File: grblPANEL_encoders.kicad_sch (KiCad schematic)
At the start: 28 parts, among them J701 Conn_01x04, J702 Conn_01x04, J703 Conn_01x04, J704 Conn_01x04

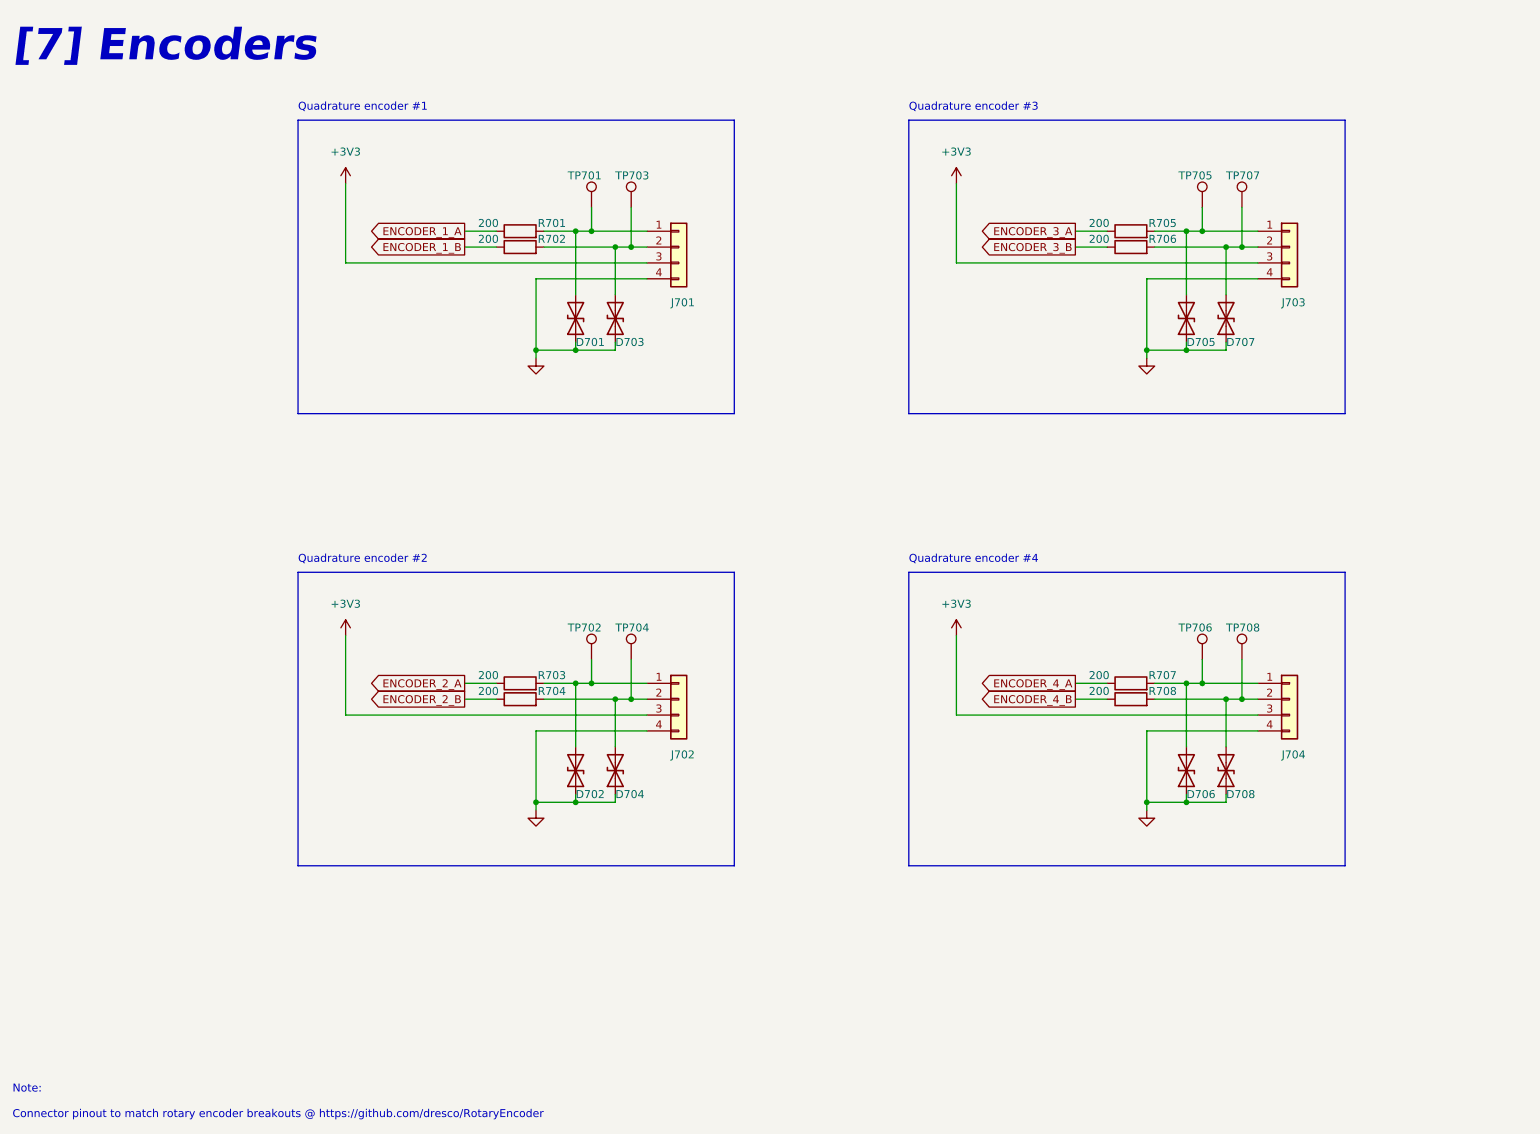
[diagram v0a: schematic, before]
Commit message: PCB layout - WIP
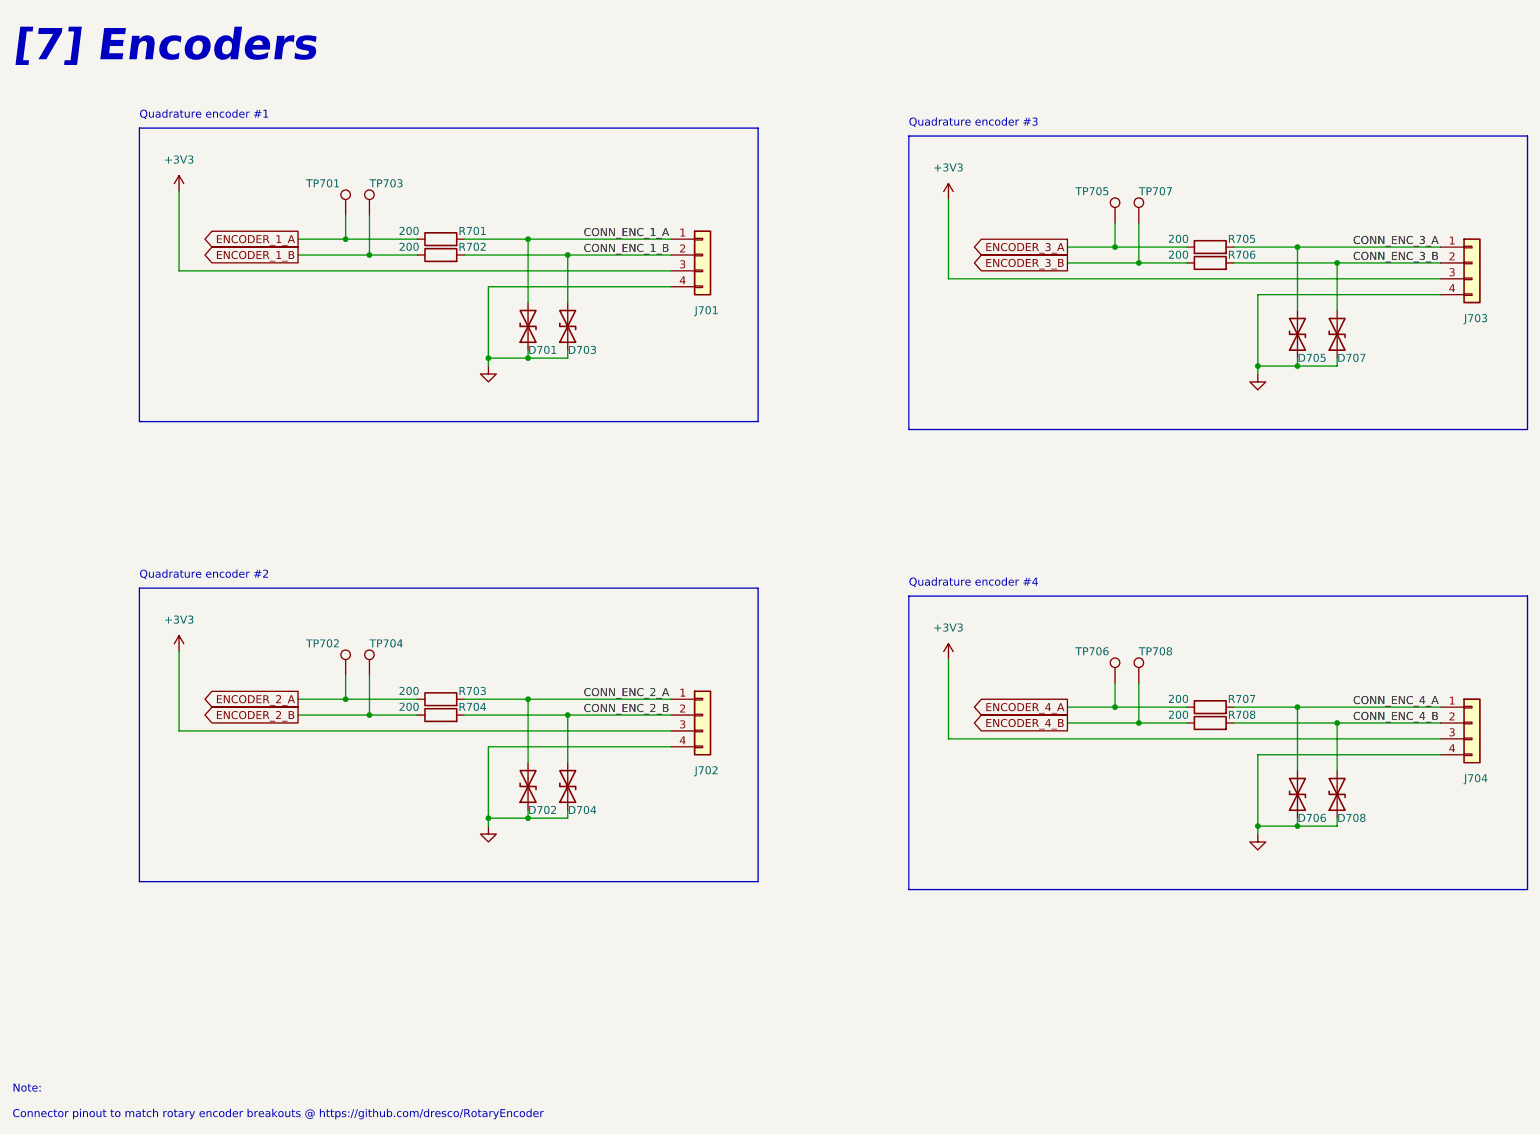
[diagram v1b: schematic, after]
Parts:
- J701, J702, J703, J704: footprint TerminalBlock_4Ucon:TerminalBlock_4Ucon_1x04_P3.50mm_Horizontal -> TerminalBlock_Phoenix:TerminalBlock_Phoenix_PT-1,5-4-3.5-H_1x04_P3.50mm_Horizontal
- TP701, TP702, TP703, TP704, TP705, TP706, TP707, TP708: footprint Connector_Pin:Pin_D1.0mm_L10.0mm -> TestPoint:TestPoint_THTPad_D2.0mm_Drill1.0mm
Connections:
- net ENCODER_1_A: now also TP701.1
- net ENCODER_1_B: now also TP703.1
- net ENCODER_2_A: now also TP702.1
- net ENCODER_2_B: now also TP704.1
- net ENCODER_3_A: now also TP705.1
- net ENCODER_3_B: now also TP707.1
- net ENCODER_4_A: now also TP706.1
- net ENCODER_4_B: now also TP708.1
- net CONN_ENC_1_B: now reaches D703.2 (A2), J701.2 (Pin_2), R702.2
- net CONN_ENC_1_B: no longer TP703.1
- net CONN_ENC_2_B: now reaches D704.2 (A2), J702.2 (Pin_2), R704.2
- net CONN_ENC_2_B: no longer TP704.1
- net CONN_ENC_3_A: now reaches D705.2 (A2), J703.1 (Pin_1), R705.2
- net CONN_ENC_3_A: no longer TP705.1
- net CONN_ENC_2_A: now reaches D702.2 (A2), J702.1 (Pin_1), R703.2
- net CONN_ENC_2_A: no longer TP702.1
- net CONN_ENC_1_A: now reaches D701.2 (A2), J701.1 (Pin_1), R701.2
- net CONN_ENC_1_A: no longer TP701.1
- net CONN_ENC_3_B: now reaches D707.2 (A2), J703.2 (Pin_2), R706.2
- net CONN_ENC_3_B: no longer TP707.1
- net CONN_ENC_4_A: now reaches D706.2 (A2), J704.1 (Pin_1), R707.2
- net CONN_ENC_4_A: no longer TP706.1
- net CONN_ENC_4_B: now reaches D708.2 (A2), J704.2 (Pin_2), R708.2
- net CONN_ENC_4_B: no longer TP708.1
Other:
- moved on the sheet: D701, D703, J701, R701, R702, TP701, TP703
